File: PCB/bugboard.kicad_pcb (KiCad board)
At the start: 2 copper layers, 20.9 x 52.3 mm, 28 parts, among them J1 USB_C_Receptacle_USB2.0_16P, J2 Conn_01x04, J3 Conn_01x20, J4 Conn_01x20, SW1 SW_SPST, SW2 SW_SPST, U1 STM32G431CBTx, U2 XC6206PxxxMR

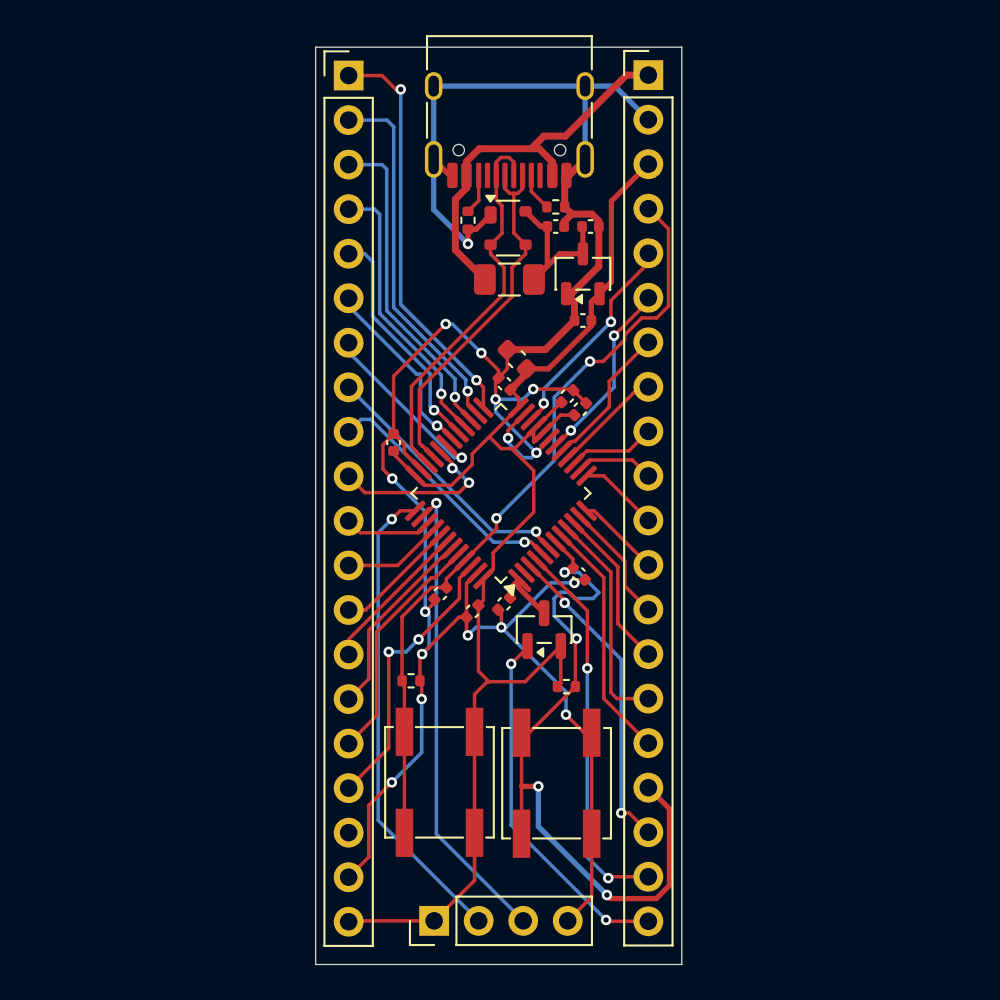
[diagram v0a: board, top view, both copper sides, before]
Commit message: Added PCB and Schematic
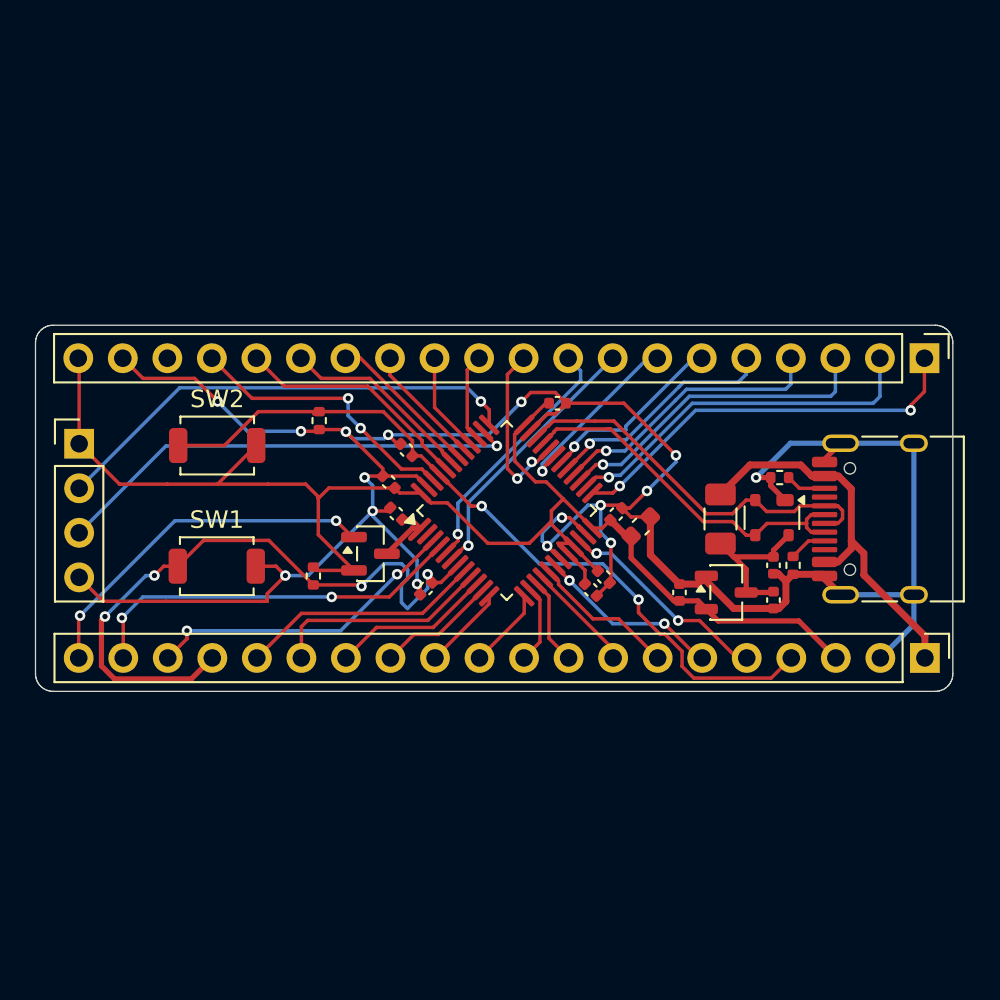
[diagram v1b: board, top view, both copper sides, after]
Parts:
- SW1, SW2: footprint Button_Switch_SMD:SW_SPST_EVPBF -> Button_Switch_SMD:SW_SPST_TS-1088-xR020
- moved J3 36.8 mm to (194.5, 84.7), turned to -90 degrees
- moved J4 36.6 mm to (194.5, 67.6), turned to -90 degrees
- moved J2 33.9 mm to (146.3, 72.5), turned to 0 degrees
- moved J1 32.3 mm to (192.9, 76.8), turned to 90 degrees
- moved R1 24.5 mm to (187.0, 79.4), turned to -90 degrees
- moved C1 23.7 mm to (185.9, 81.4), turned to -90 degrees
- moved R2 23.1 mm to (186.3, 74.4), turned to 0 degrees
- moved SW2 23.0 mm to (154.2, 72.6), turned to 0 degrees
- moved SW1 23.0 mm to (154.2, 79.5), turned to 0 degrees
- moved C11 23.0 mm to (185.9, 79.4), turned to -90 degrees
- moved D2 22.3 mm to (185.8, 76.7), turned to -90 degrees
- moved U2 19.9 mm to (183.2, 81.0), turned to 0 degrees
- moved F1 18.2 mm to (182.9, 76.8), turned to -90 degrees
- moved C2 16.5 mm to (180.5, 81.0), turned to -90 degrees
- moved R3 15.8 mm to (159.7, 80.0), turned to -90 degrees
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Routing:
- net NRST: track 42.3 -> 38.3 mm
- net +3V3: track 80.4 -> 83.5 mm
- net GND: track 147.1 -> 149.0 mm
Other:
- board size 20.9 x 52.3 mm -> 52.3 x 20.9 mm
